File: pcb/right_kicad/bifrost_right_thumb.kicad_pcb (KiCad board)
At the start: 2 copper layers, 44.8 x 20.8 mm, 9 parts, among them J1 Conn_01x05, SW1 1U, SW2 1U

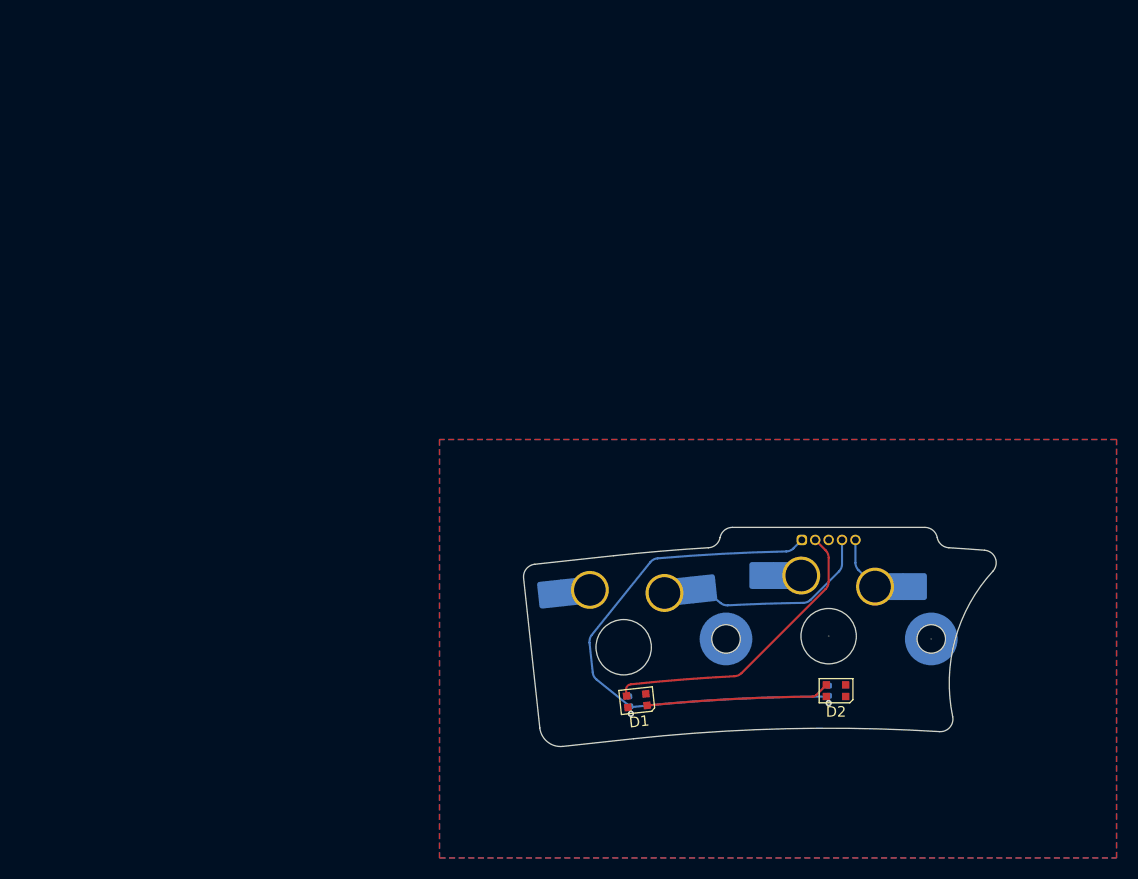
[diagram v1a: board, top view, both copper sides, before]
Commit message: Update PCB and case designs
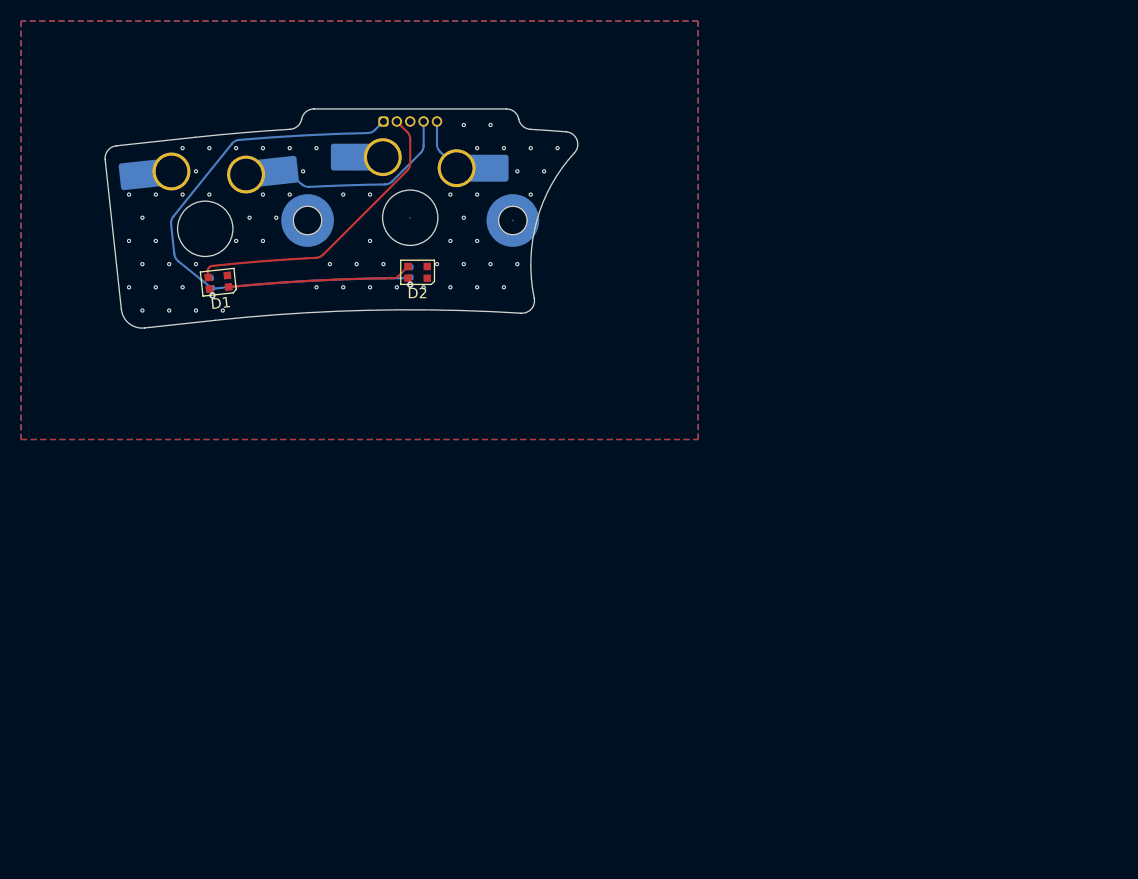
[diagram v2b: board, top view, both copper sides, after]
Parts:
- moved H2 56.1 mm to (109.0, 59.8)
- moved J1 56.1 mm to (96.7, 50.4)
- moved C1 56.1 mm to (80.3, 65.7)
- moved C2 56.1 mm to (99.2, 64.7)
- moved D1 56.1 mm to (81.0, 65.6)
- moved SW2 56.1 mm to (99.2, 59.5)
- moved D2 56.1 mm to (99.9, 64.7)
- moved H1 56.1 mm to (89.5, 59.8)
- moved SW1 56.1 mm to (79.8, 60.6)
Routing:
- net GND: vias 0 -> 63
